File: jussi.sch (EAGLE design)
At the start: 3 parts

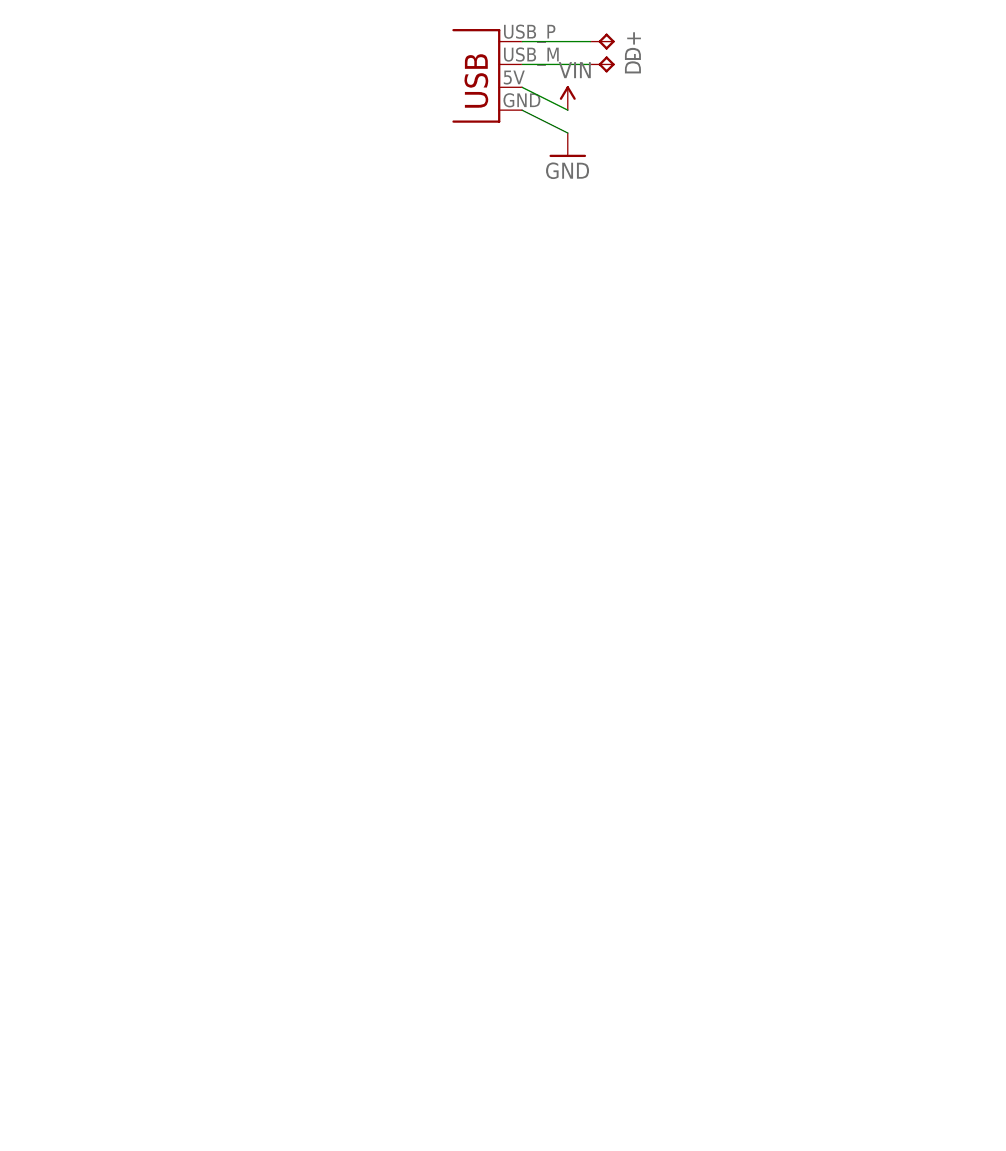
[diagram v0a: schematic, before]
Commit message: "Done"
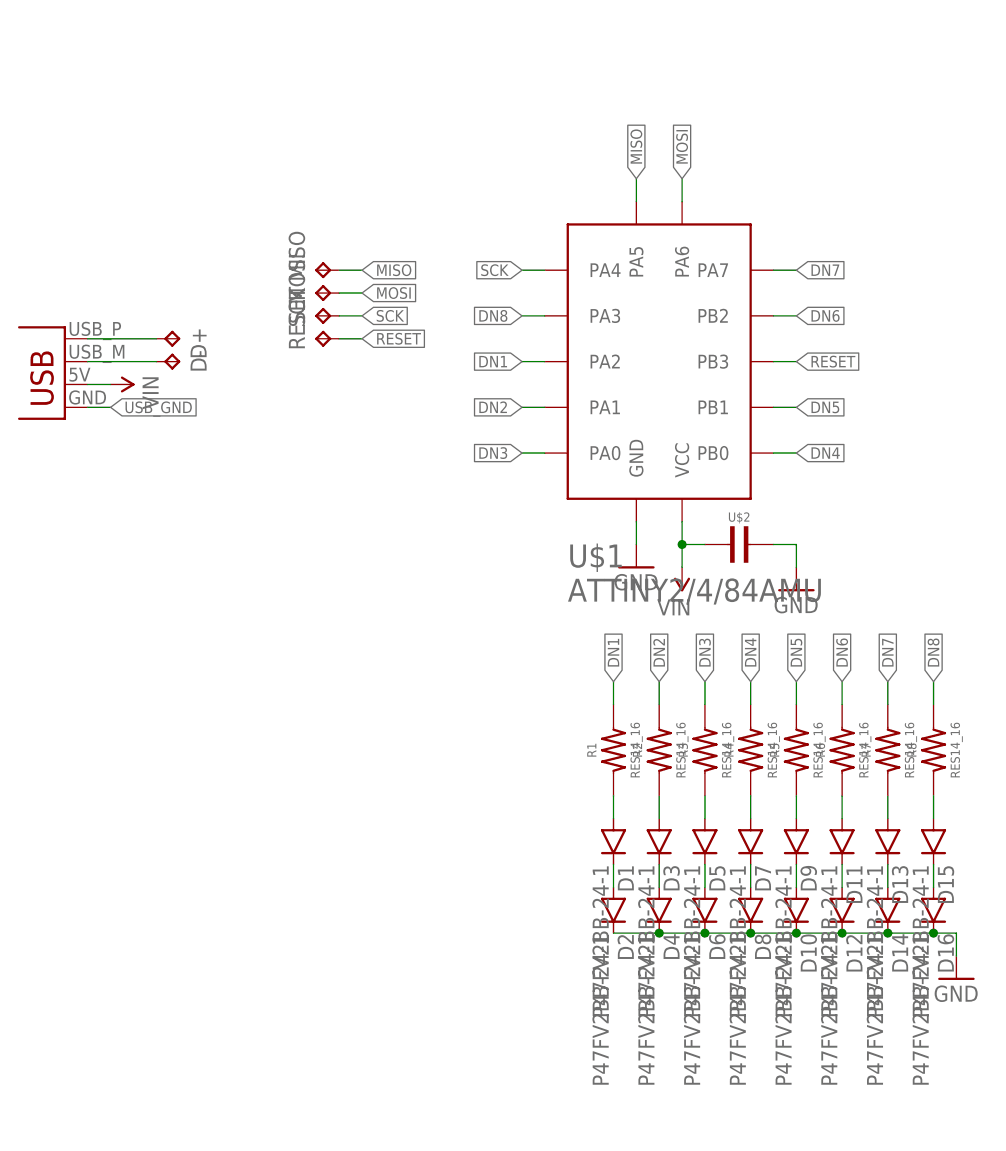
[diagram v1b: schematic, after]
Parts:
- added D1, D10, D11, D12, D13, D14, D15, D16, D2, D3, D4, D5, D6, D7, D8, D9: P47FV2BB-24-1, pcb-card:P47FV2BB-24-1
- added MISO, MOSI, RESET, SCK: TPTP08R, testpad:TPTP08R
- added R1, R2, R3, R4, R5, R6, R7, R8: RES14_16, dubec:RES14_16
- added U$1: ATTINY2/4/84AMU, pcb-card:ATTINY2/4/84AMU
- added U$2: (no value), dubec:CAP47UF_10V
- D+, D-: value TPTP06R -> TPTP08R; device testpad:TPTP06R -> testpad:TPTP08R
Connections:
- new net DN1: R1.2, U$1.PA2
- new net DN2: R2.2, U$1.PA1
- new net DN3: R3.2, U$1.PA0
- new net DN4: R4.2, U$1.PB0
- new net DN5: R5.2, U$1.PB1
- new net DN6: R6.2, U$1.PB2
- new net DN7: R7.2, U$1.PA7
- new net DN8: R8.2, U$1.PA3
- new net MISO: MISO.TP, U$1.PA5
- new net MOSI: MOSI.TP, U$1.PA6
- new net N$1: D1.C, D2.A
- new net N$10: D3.A, R2.1
- new net N$11: D5.A, R3.1
- new net N$12: D7.A, R4.1
- new net N$13: D9.A, R5.1
- new net N$14: D11.A, R6.1
- new net N$15: D13.A, R7.1
- new net N$16: D15.A, R8.1
- new net N$2: D3.C, D4.A
- new net N$3: D5.C, D6.A
- new net N$4: D7.C, D8.A
- new net N$5: D10.A, D9.C
- new net N$6: D11.C, D12.A
- new net N$7: D13.C, D14.A
- new net N$8: D15.C, D16.A
- new net N$9: D1.A, R1.1
- new net RESET: RESET.TP, U$1.PB3
- new net SCK: SCK.TP, U$1.PA4
- new net USB_GND: JP1.GND
- net GND: now also D10.C, D12.C, D14.C, D16.C, D2.C, D4.C, D6.C, D8.C, U$1.GND, U$2.2; no longer JP1.GND
- net VIN: now also U$1.VCC, U$2.1
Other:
- moved on the sheet: D+, D-

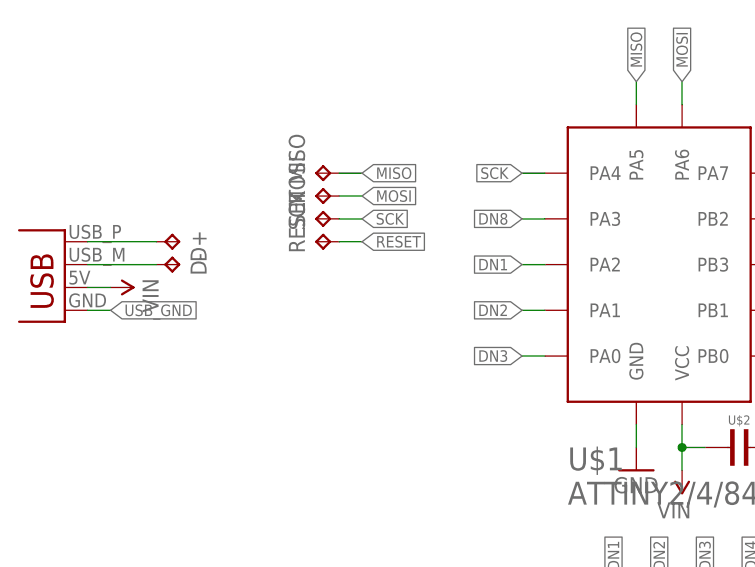
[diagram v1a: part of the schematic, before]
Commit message: Zip generated
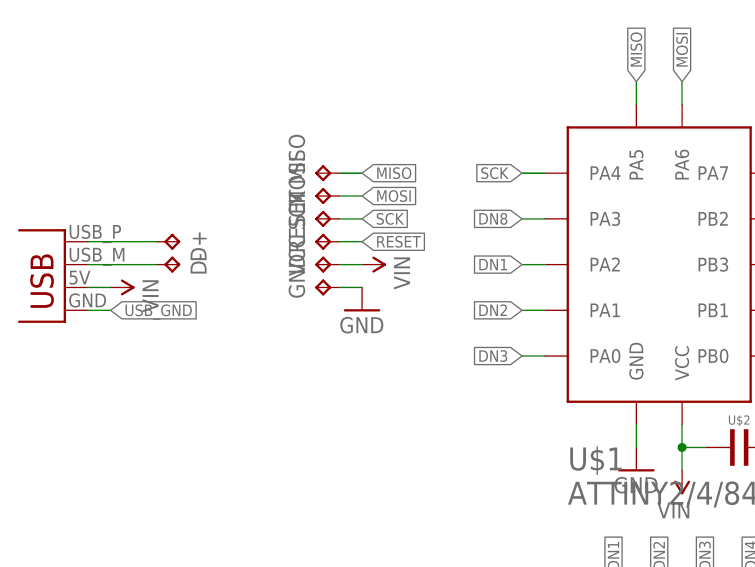
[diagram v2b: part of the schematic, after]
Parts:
- added GND, VCC: TPTP08R, testpad:TPTP08R
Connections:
- net GND: now also GND.TP
- net VIN: now also VCC.TP
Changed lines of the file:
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@@
 <part name="SCK" library="testpad" deviceset="TP" device="TP08R" value="TPTP08R"/>
 <part name="RESET" library="testpad" deviceset="TP" device="TP08R" value="TPTP08R"/>
+<part name="VCC" library="testpad" deviceset="TP" device="TP08R" value="TPTP08R"/>
+<part name="GND" library="testpad" deviceset="TP" device="TP08R" value="TPTP08R"/>
+<part name="SUPPLY3" library="SparkFun-Aesthetics" deviceset="VIN" device=""/>
+<part name="GND4" library="SparkFun-Aesthetics" deviceset="GND" device=""/>
 </parts>
 <sheets>
@@
 <instance part="SCK" gate="G$1" x="-17.78" y="48.26" rot="R90"/>
 <instance part="RESET" gate="G$1" x="-17.78" y="45.72" rot="R90"/>
+<instance part="VCC" gate="G$1" x="-17.78" y="43.18" rot="R90"/>
+<instance part="GND" gate="G$1" x="-17.78" y="40.64" rot="R90"/>
+<instance part="SUPPLY3" gate="G$1" x="-12.7" y="43.18" rot="R270"/>
+<instance part="GND4" gate="1" x="-12.7" y="38.1"/>
 </instances>
 <busses>
@@
 <wire x1="22.86" y1="22.86" x2="25.4" y2="22.86" width="0.1524" layer="91"/>
 <junction x="22.86" y="22.86"/>
+</segment>
+<segment>
+<pinref part="VCC" gate="G$1" pin="TP"/>
+<wire x1="-15.24" y1="43.18" x2="-12.7" y2="43.18" width="0.1524" layer="91"/>
+<pinref part="SUPPLY3" gate="G$1" pin="VIN"/>
 </segment>
 </net>
@@
 <pinref part="GND3" gate="1" pin="GND"/>
 </segment>
-</net>
+<segment>
+<pinref part="GND" gate="G$1" pin="TP"/>
+<wire x1="-15.24" y1="40.64" x2="-12.7" y2="40.64" width="0.1524" layer="91"/>
+<pinref part="GND4" gate="1" pin="GND"/>
+</segment>
+</net>
